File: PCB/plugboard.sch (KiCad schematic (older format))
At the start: 121 parts, among them J1 1/4\" Jack, J10 Conn_01x19_Male_0, J11 Conn_01x19_Male_0, J2 1/4\" Jack, J3 1/4\" Jack, J4 1/4\" Jack, J5 1/4\" Jack, J6 1/4\" Jack, J7 1/4\" Jack, J8 1/4\" Jack, J9 1/4\" Jack, P1 CONN_02X03, P2 CONN_02X03, U1 ADG732

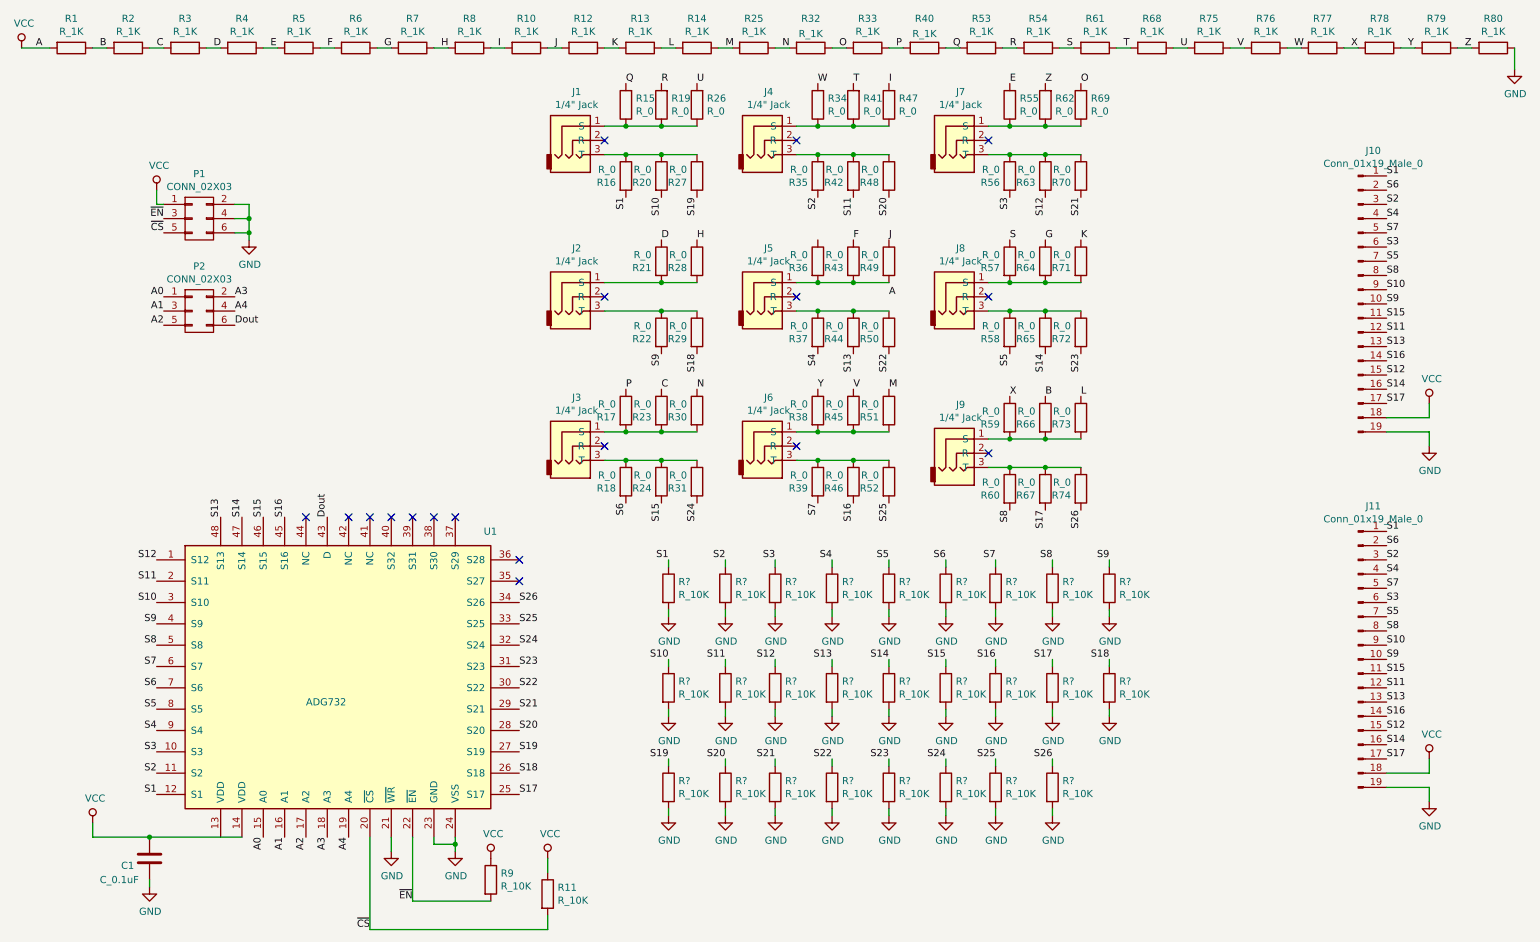
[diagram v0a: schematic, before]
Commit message: Basic Layout
Now I'm gonna start on tracing.
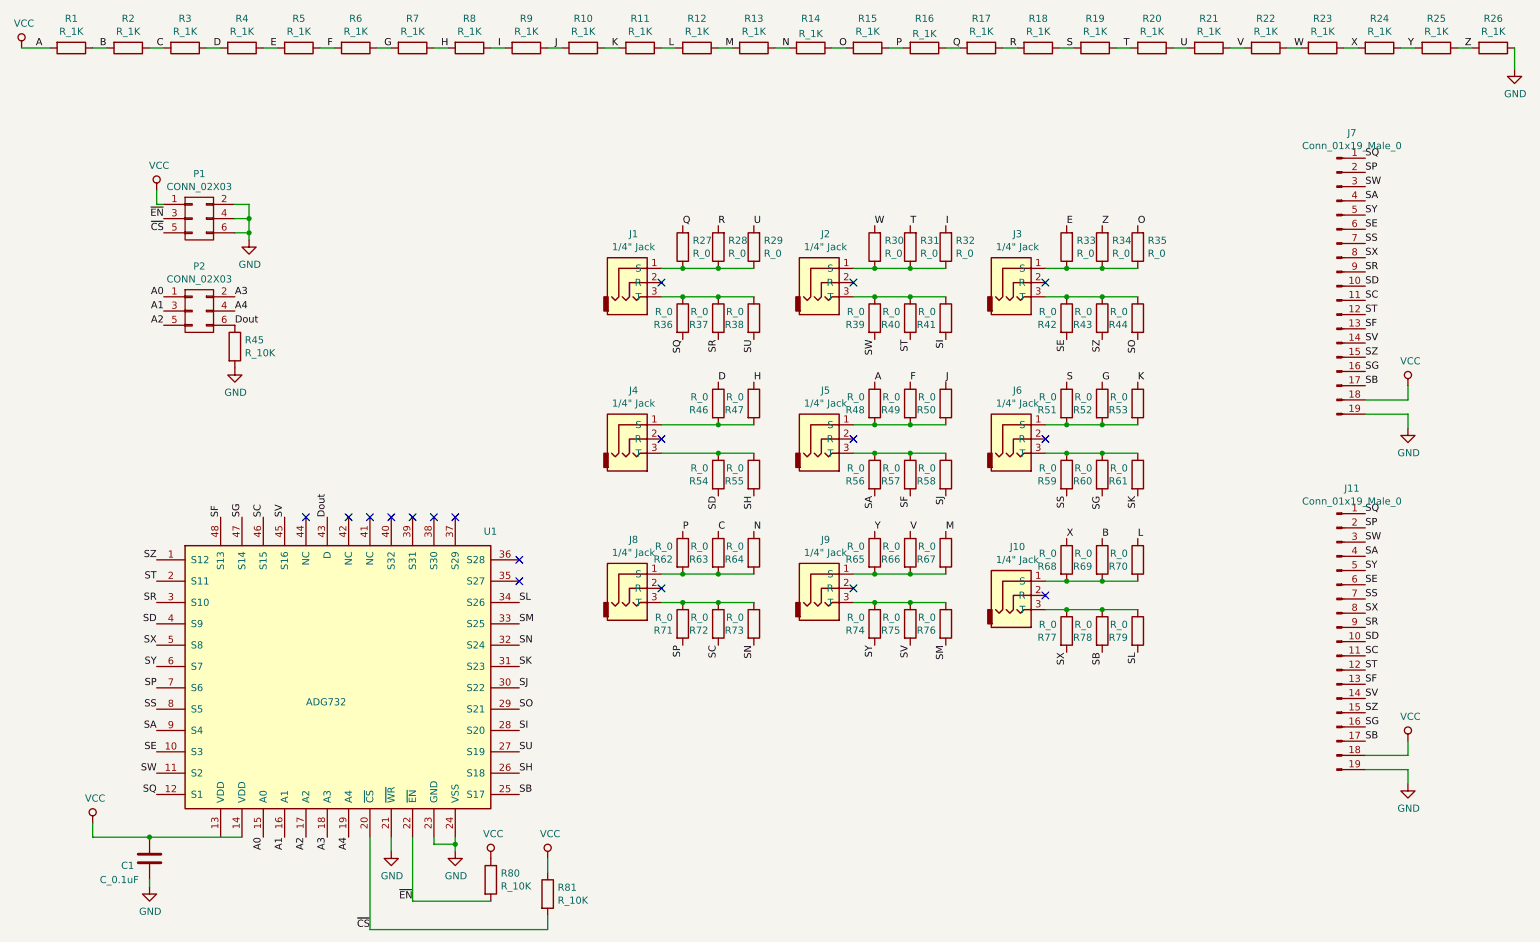
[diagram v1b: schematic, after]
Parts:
- removed R? (x26): R_10K, enigmaprints:R_0805_OEM, symbol formula:R_10K
- added R45: R_10K, enigmaprints:R_0805_OEM, symbol formula:R_10K
- C1: footprint footprints:C_0805_OEM -> enigmaprints:R_0805_OEM
- U1: footprint footprints:48-TQFP -> enigmaprints:ADG732BSUZ-REEL
- renumbered J9 to J10, J4 to J2, J7 to J3, J2 to J4, J8 to J6, J10 to J7, J3 to J8, J6 to J9, R12 to R10, R13 to R11, R14 to R12, R25 to R13, R32 to R14, R33 to R15, R40 to R16, R53 to R17, R54 to R18, R61 to R19, R68 to R20, R75 to R21, R76 to R22, R77 to R23, R78 to R24, R79 to R25, R80 to R26, R15 to R27, R19 to R28, R26 to R29, R34 to R30, R41 to R31, R47 to R32, R55 to R33, R62 to R34, R69 to R35, R16 to R36, R20 to R37, R27 to R38, R35 to R39, R42 to R40, R48 to R41, R56 to R42, R63 to R43, R70 to R44, R21 to R46, R28 to R47, R36 to R48, R43 to R49, R49 to R50, R57 to R51, R64 to R52, R71 to R53, R22 to R54, R29 to R55, R37 to R56, R44 to R57, R50 to R58, R58 to R59, R65 to R60, R72 to R61, R17 to R62, R23 to R63, R30 to R64, R38 to R65, R45 to R66, R51 to R67, R59 to R68, R66 to R69, R73 to R70, R18 to R71, R24 to R72, R31 to R73, R39 to R74, R46 to R75, R52 to R76, R60 to R77, R67 to R78, R74 to R79, R9 to R80, R11 to R81, R10 to R9
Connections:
- net Dout: now also R45.1
- net GND: now also R45.2
- net VCC: now also R48.1
- net S1 renamed SQ
- net S10 renamed SR
- net S11 renamed ST
- net S12 renamed SZ
- net S13 renamed SF
- net S14 renamed SG
- net S15 renamed SC
- net S16 renamed SV
- net S17 renamed SB
- net S18 renamed SH
- net S19 renamed SU
- net S2 renamed SW
- net S20 renamed SI
- net S21 renamed SO
- net S22 renamed SJ
- net S23 renamed SK
- net S24 renamed SN
- net S25 renamed SM
- net S26 renamed SL
- net S3 renamed SE
- net S4 renamed SA
- net S5 renamed SS
- net S6 renamed SP
- net S7 renamed SY
- net S8 renamed SX
- net S9 renamed SD
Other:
- moved on the sheet: J1, J10, J11, J2, J3, J4, J5, J6, J7, J8, J9, R27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
